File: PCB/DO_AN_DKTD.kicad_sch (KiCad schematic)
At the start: 0 parts

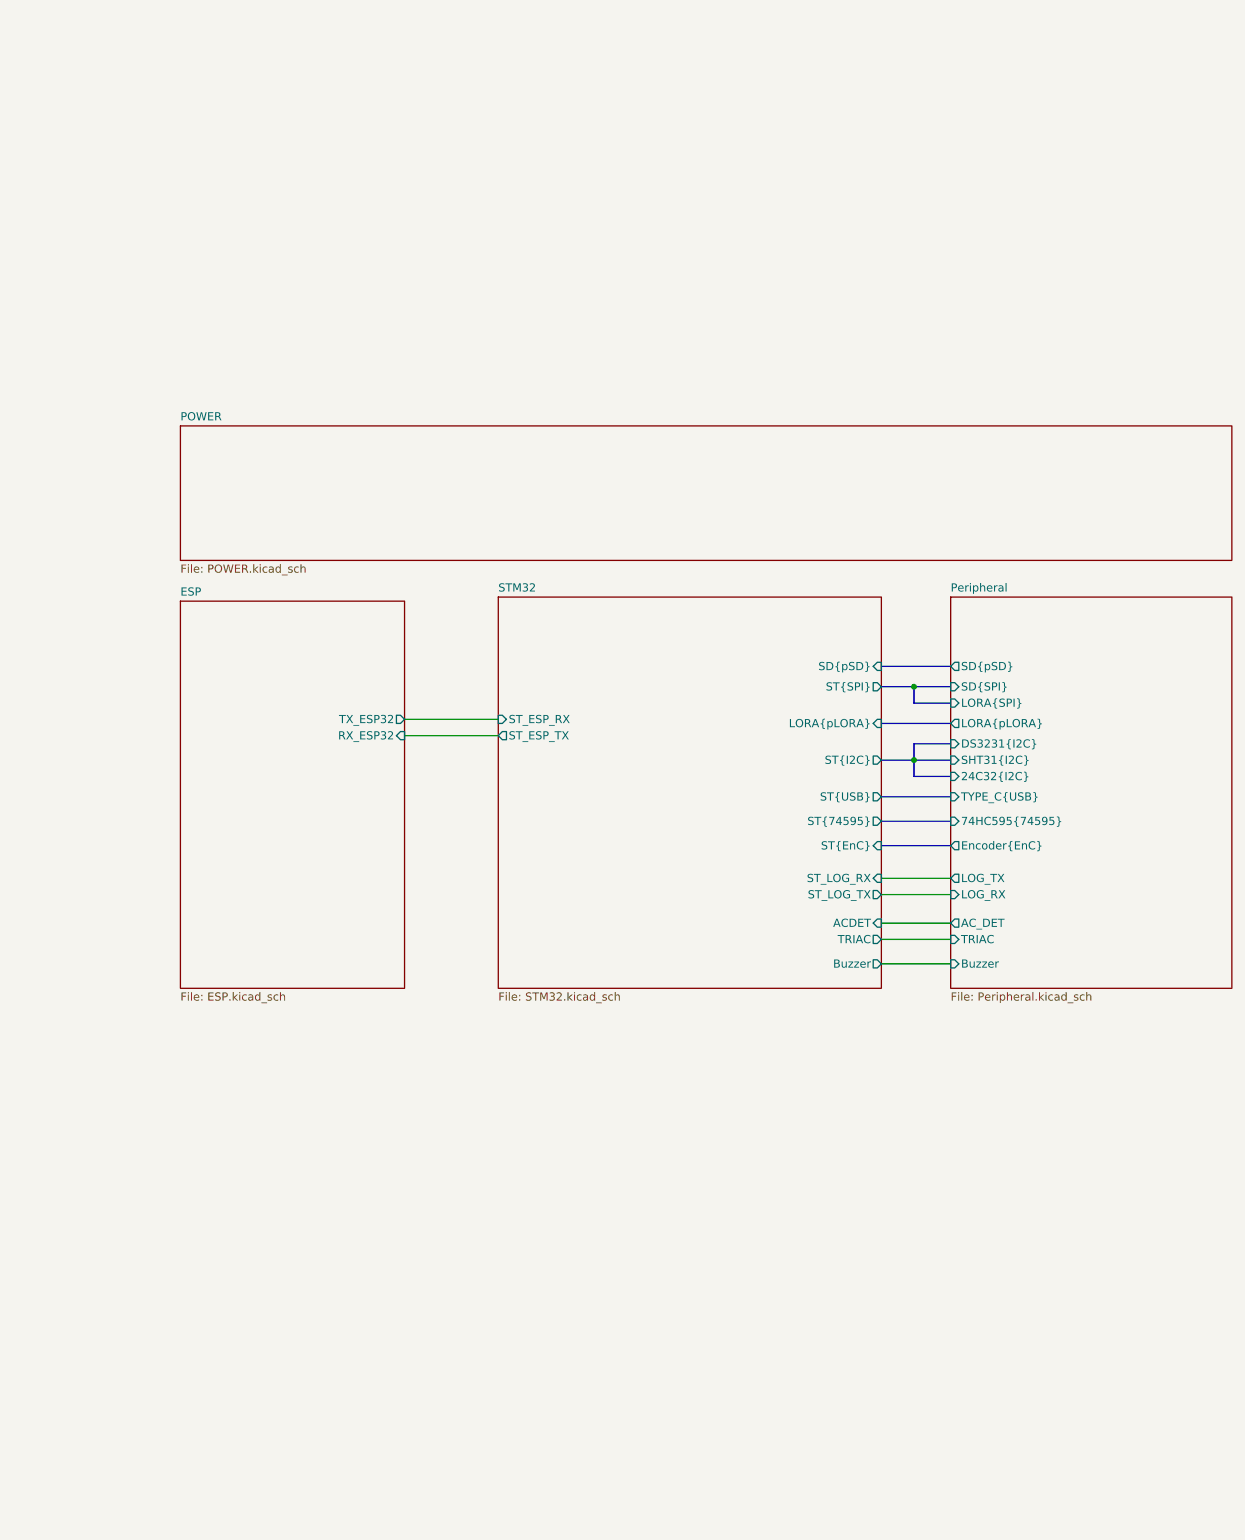
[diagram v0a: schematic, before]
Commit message: raw placement
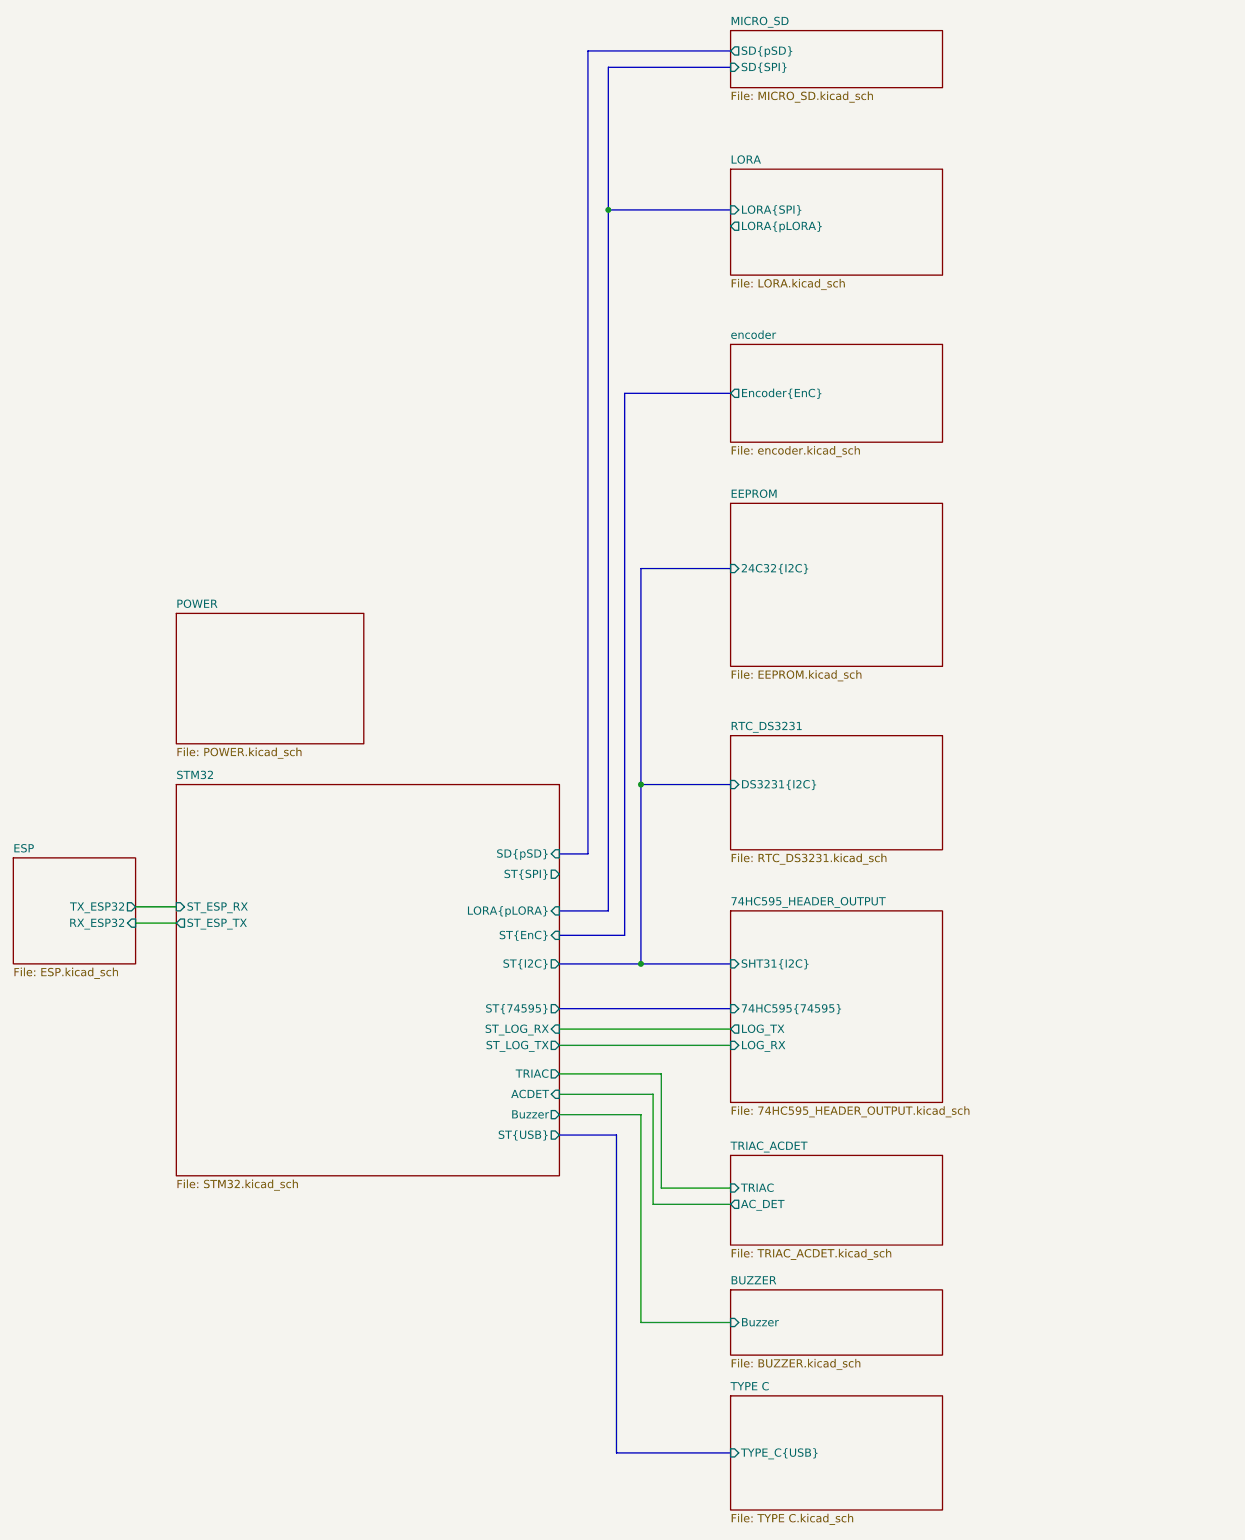
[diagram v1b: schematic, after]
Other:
- sheet Peripheral renamed 74HC595_HEADER_OUTPUT
- added sheet BUZZER (BUZZER.kicad_sch)
- added sheet EEPROM (EEPROM.kicad_sch)
- added sheet LORA (LORA.kicad_sch)
- added sheet MICRO_SD (MICRO_SD.kicad_sch)
- added sheet RTC_DS3231 (RTC_DS3231.kicad_sch)
- added sheet TRIAC_ACDET (TRIAC_ACDET.kicad_sch)
- added sheet TYPE C (TYPE C.kicad_sch)
- added sheet encoder (encoder.kicad_sch)
- sheet 74HC595_HEADER_OUTPUT: file Peripheral.kicad_sch -> 74HC595_HEADER_OUTPUT.kicad_sch
- sheet 74HC595_HEADER_OUTPUT ports: added none; removed 24C32{I2C}, AC_DET, Buzzer, DS3231{I2C}, Encoder{EnC}, LORA{SPI}, LORA{pLORA}, SD{SPI}, SD{pSD}, TRIAC, TYPE_C{USB}
